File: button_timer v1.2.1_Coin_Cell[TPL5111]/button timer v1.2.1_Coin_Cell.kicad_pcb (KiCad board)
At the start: 2 copper layers, 21 x 47.8 mm, 25 parts, among them J1 Conn_01x05_Female, Q1 TSM2323, SW1 SW_Push, SW2 SW_Push, U1 TPS61097A, U2 TPL5110, X1 ESP-12E

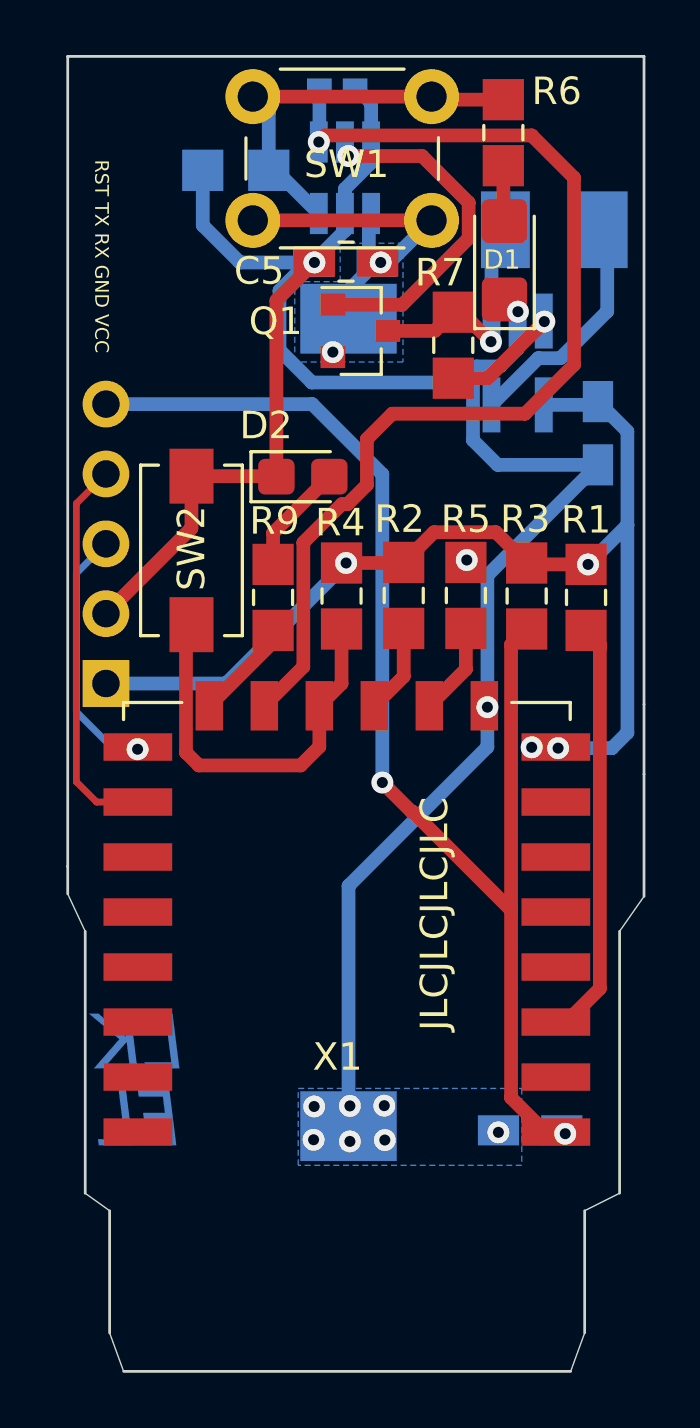
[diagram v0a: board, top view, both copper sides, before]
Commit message: :rocket: :full_moon_with_face:
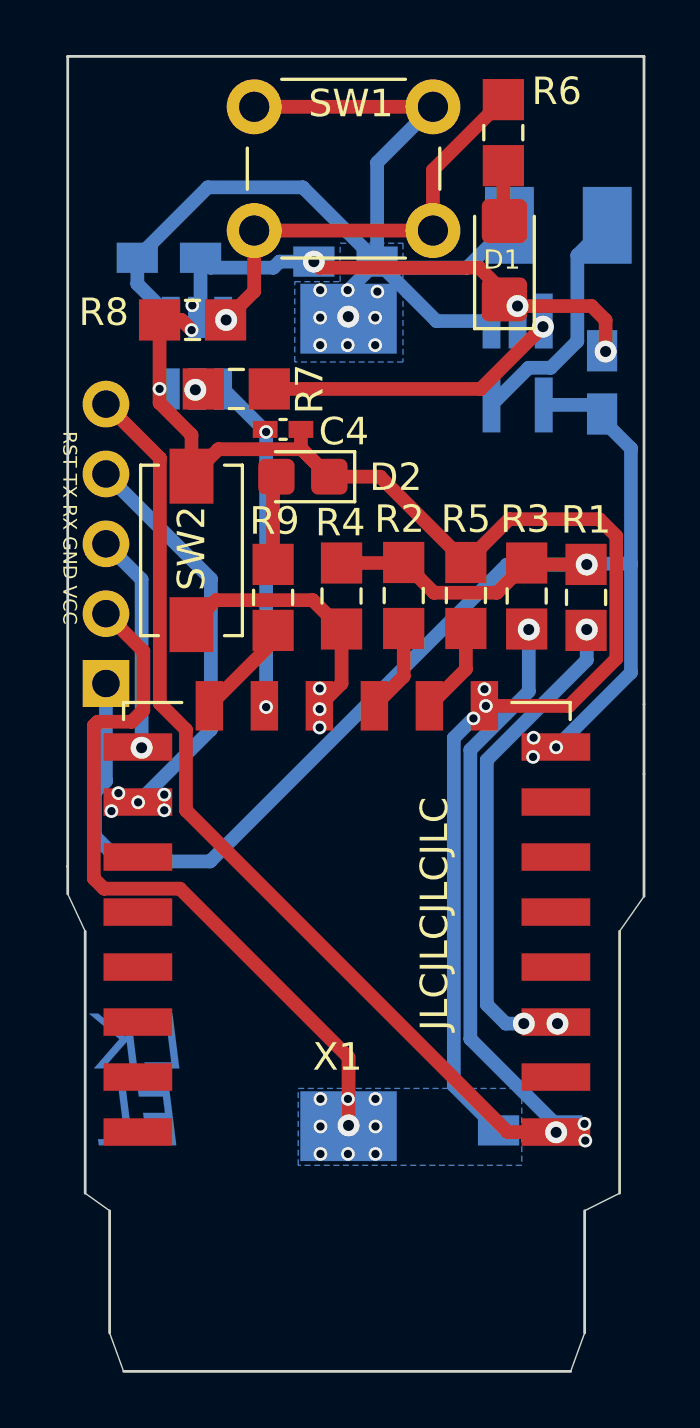
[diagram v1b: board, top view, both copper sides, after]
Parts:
- removed Q1: TSM2323, Package_TO_SOT_SMD:SOT-23
- removed U2: TPL5110, handsolder:SOT-23-6handsoldering
- added U3: TPL5111, handsolder:SOT-23-6handsoldering, B.Cu at (120.3, 65.3)
- C4, R8: moved to F.Cu
- C5: moved to B.Cu
- moved C4 12.6 mm to (123.4, 68.1)
- moved R7 8.05 mm to (121.7, 66.6), turned to 0 degrees
- moved SW1 7.66 mm to (122.3, 56.4), turned to 0 degrees
- moved C5 6.44 mm to (119.2, 61.9), turned to 180 degrees
- moved R8 5.66 mm to (120.1, 64.1)
- moved C3 1.86 mm to (135.0, 66.4), turned to 90 degrees
- moved L1 0.22 mm to (133.4, 60.7)
- turned D2 to 180 degrees
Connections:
- L1 pad 1: Net-(L1-Pad1) -> Net-(BT1-Pad1)
- R7 pad 2: Net-(L1-Pad1) -> Net-(R7-Pad2)
- U1 pad 1: Net-(L1-Pad1) -> Net-(BT1-Pad1)
- U1 pad 3: Net-(R7-Pad1) -> Net-(R7-Pad2)
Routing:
- net /GPIO4: track 38.8 -> 12.2 mm, vias 1 -> 2
- net Net-(BT1-Pad1): track 13.5 -> 39.6 mm, vias 2 -> 9
- net /GND: track 82.7 -> 99.7 mm, vias 11 -> 18
- net /VCC: track 39.7 -> 55.9 mm
- net Net-(Q1-Pad1): track 12.3 -> 0.00 mm, vias 1 -> 0
- net Net-(R7-Pad2): track 0.00 -> 10.9 mm, vias 0 -> 1
- net Net-(L1-Pad1): track 8.00 -> 0.00 mm, vias 1 -> 0
- net /RST: track 48.7 -> 54.7 mm, vias 2 -> 4
- net /GPIO0: track 14.7 -> 9.39 mm, vias 0 -> 3
- net Net-(R7-Pad1): track 4.16 -> 0.00 mm
- net /EN: track 15.3 -> 18.0 mm, vias 0 -> 3
- net Net-(R6-Pad2): track 14.5 -> 16.0 mm, vias 0 -> 1
- net /RX: track 9.34 -> 7.95 mm
- net Net-(D2-Pad2): track 4.04 -> 3.24 mm
- net /TX: track 14.2 -> 14.6 mm, vias 0 -> 5
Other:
- board text added: "V.1.2.1 ONLY COIN CELL TIMER TPL5111"
- board text removed: "V.1.2.1 ONLY COIN CELL TIMER TPL5110"
